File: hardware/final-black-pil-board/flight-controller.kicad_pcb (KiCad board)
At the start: 2 copper layers, 58.5 x 67.2 mm, 29 parts, among them IC1 BMI088, IC2 BMP390, J1 Conn_01x04, J2 Conn_01x04, J3 Conn_02x04_Odd_Even, J4 Conn_01x09, J5 Conn_02x08_Odd_Even, J6 Conn_02x04_Odd_Even, J8 RASPBERRY_PI_4B_+_Samtec_ESP-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, U1 PCA9685BS

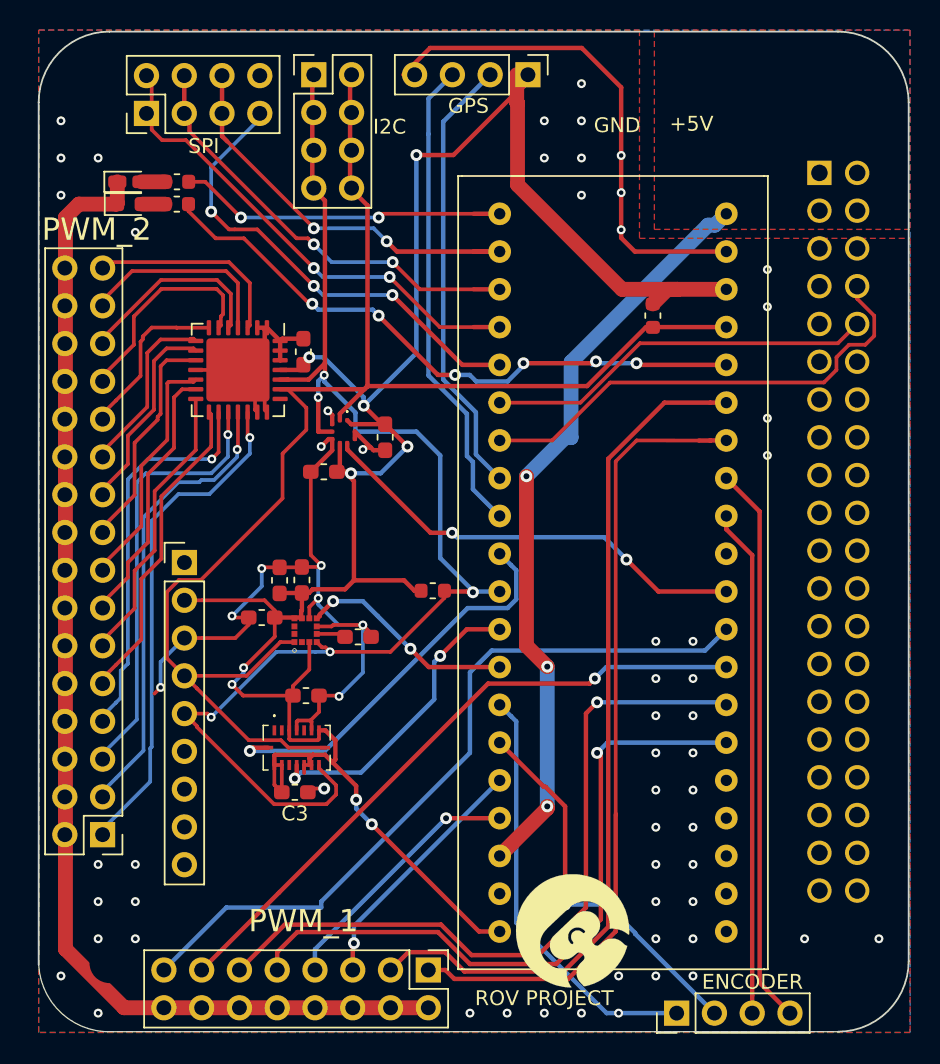
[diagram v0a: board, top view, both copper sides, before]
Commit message: UART communication
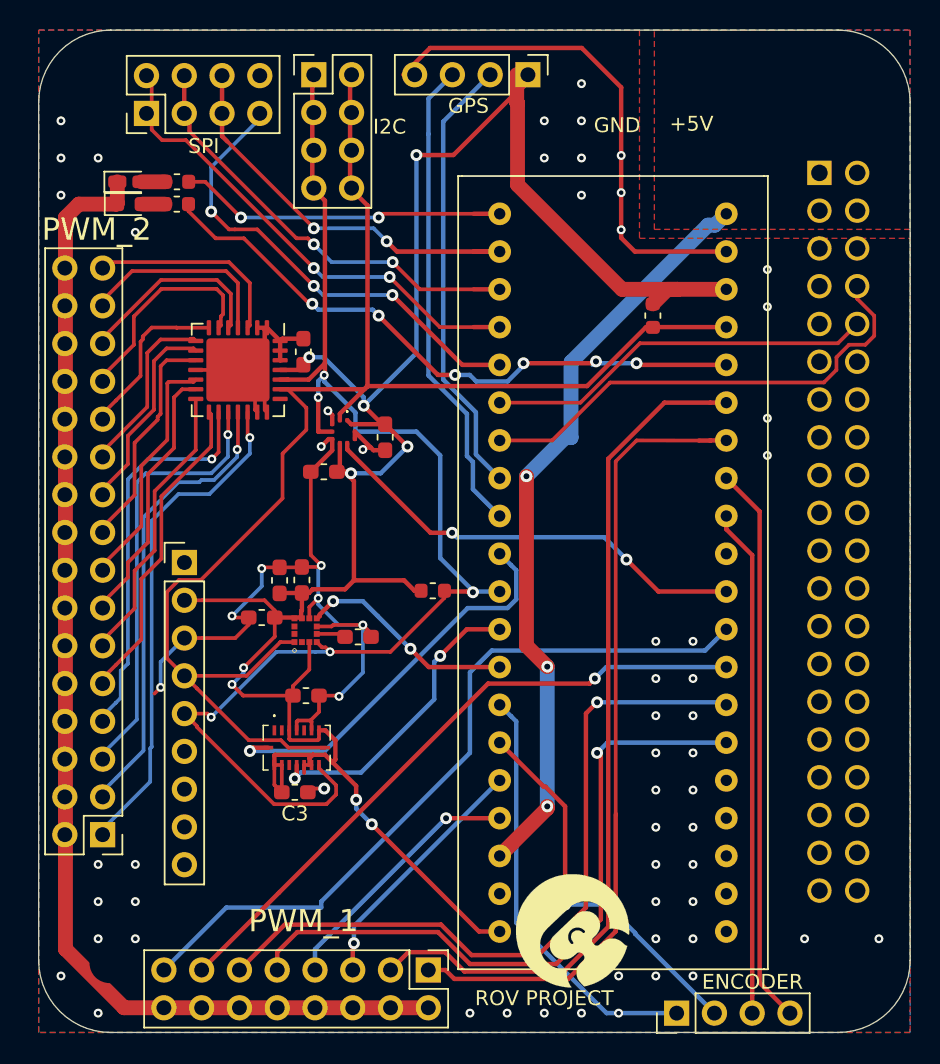
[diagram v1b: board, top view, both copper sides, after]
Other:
- board size 58.5 x 67.2 mm -> 58.6 x 67.4 mm
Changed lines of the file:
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@@
       (effects (font (size 1 1) (thickness 0.15)))
     )
-    (fp_text value Conn_01x04 (at 0 9.95 90) (layer F.Fab)
+    (fp_text value Conn_01x04 (at -1.2 10.85 90) (layer F.Fab)
       (effects (font (size 1 1) (thickness 0.15)))
     )
@@
     )
   )
+  (gr_line (start 144.75 108.8) (end 95.85 108.8) (layer Edge.Cuts) (width 0.05))
+  (gr_line (start 149.6 46.25) (end 149.6 103.95) (layer Edge.Cuts) (width 0.05))
+  (gr_line (start 144.75 41.4) (end 95.85 41.4) (layer Edge.Cuts) (width 0.05))
+  (gr_line (start 91 103.95) (end 91 46.25) (layer Edge.Cuts) (width 0.05))
+  (gr_arc (start 95.85 103.95) (end 91 103.95) (angle -90) (layer Edge.Cuts) (width 0.05))
+  (gr_arc (start 144.75 103.95) (end 144.75 108.8) (angle -90) (layer Edge.Cuts) (width 0.05))
+  (gr_arc (start 144.75 46.25) (end 149.6 46.25) (angle -90) (layer Edge.Cuts) (width 0.05))
+  (gr_arc (start 95.85 46.25) (end 95.85 41.4) (angle -90) (layer Edge.Cuts) (width 0.05))
   (gr_text ENCODER (at 139 105.4) (layer F.SilkS)
     (effects (font (size 1 1) (thickness 0.15)))
@@
     (effects (font (size 1.5 1.5) (thickness 0.3)))
   )
-  (gr_line (start 95.999999 108.749999) (end 144.75 108.75) (layer Edge.Cuts) (width 0.05))
-  (gr_arc (start 95.75 104) (end 91.000001 104.249999) (angle -90) (layer Edge.Cuts) (width 0.05))
   (gr_text "ROV PROJECT" (at 125 106.5) (layer F.SilkS)
     (effects (font (size 1 1) (thickness 0.15)))
   )
-  (gr_line (start 91 46.25) (end 91 104.25) (layer Edge.Cuts) (width 0.12))
-  (gr_line (start 144.75 41.5) (end 95.75 41.5) (layer Edge.Cuts) (width 0.12))
-  (gr_line (start 149.5 104) (end 149.5 46.25) (layer Edge.Cuts) (width 0.12))
-  (gr_arc (start 144.75 104) (end 144.75 108.75) (angle -90) (layer Edge.Cuts) (width 0.12))
-  (gr_arc (start 95.75 46.25) (end 95.75 41.5) (angle -90) (layer Edge.Cuts) (width 0.12))
-  (gr_arc (start 144.75 46.25) (end 149.5 46.25) (angle -90) (layer Edge.Cuts) (width 0.12))
   (segment (start 111.25 70.9) (end 111.05 71.1) (width 0.3) (layer F.Cu) (net 3))
   (segment (start 111.25 69.163) (end 111.25 70.9) (width 0.3) (layer F.Cu) (net 3))

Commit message: softw update
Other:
- net class Default removed
